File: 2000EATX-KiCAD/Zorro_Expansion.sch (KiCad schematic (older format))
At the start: 119 parts, among them CN601 Amiga-2000-Zorro-Slot, CN602 Amiga-2000-Zorro-Slot, CN603 Amiga-2000-Zorro-Slot, CN604 Amiga-2000-Zorro-Slot, CN605 Amiga-2000-Zorro-Slot, U606 74LS32

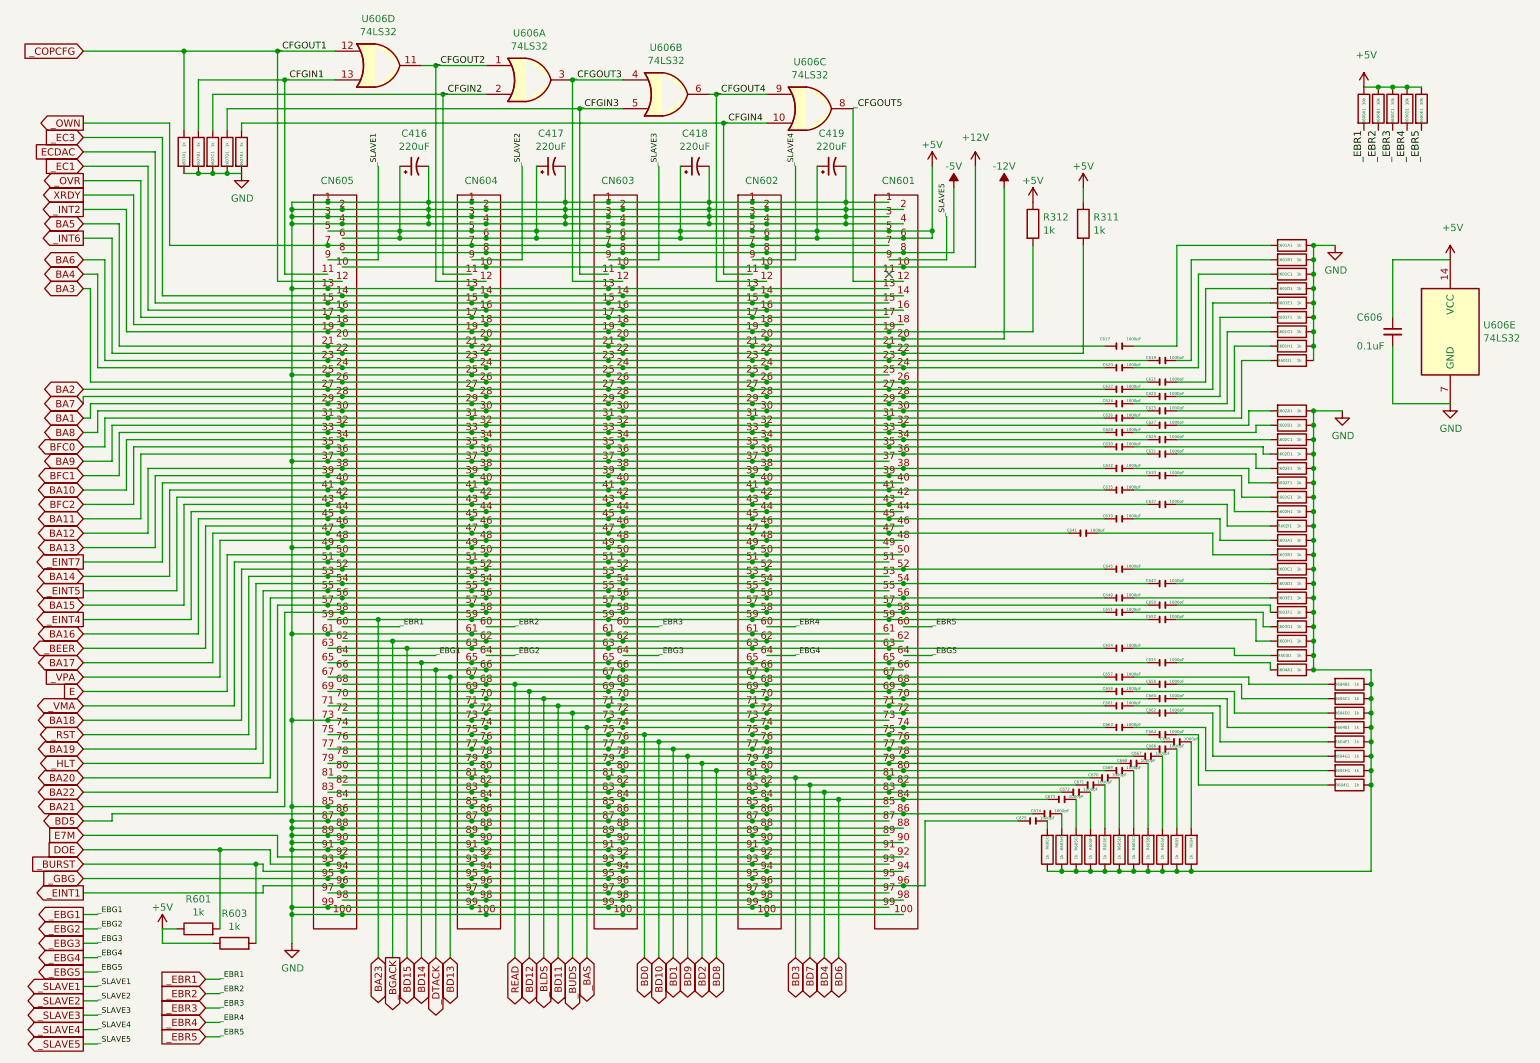
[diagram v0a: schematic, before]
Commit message: Add files via upload
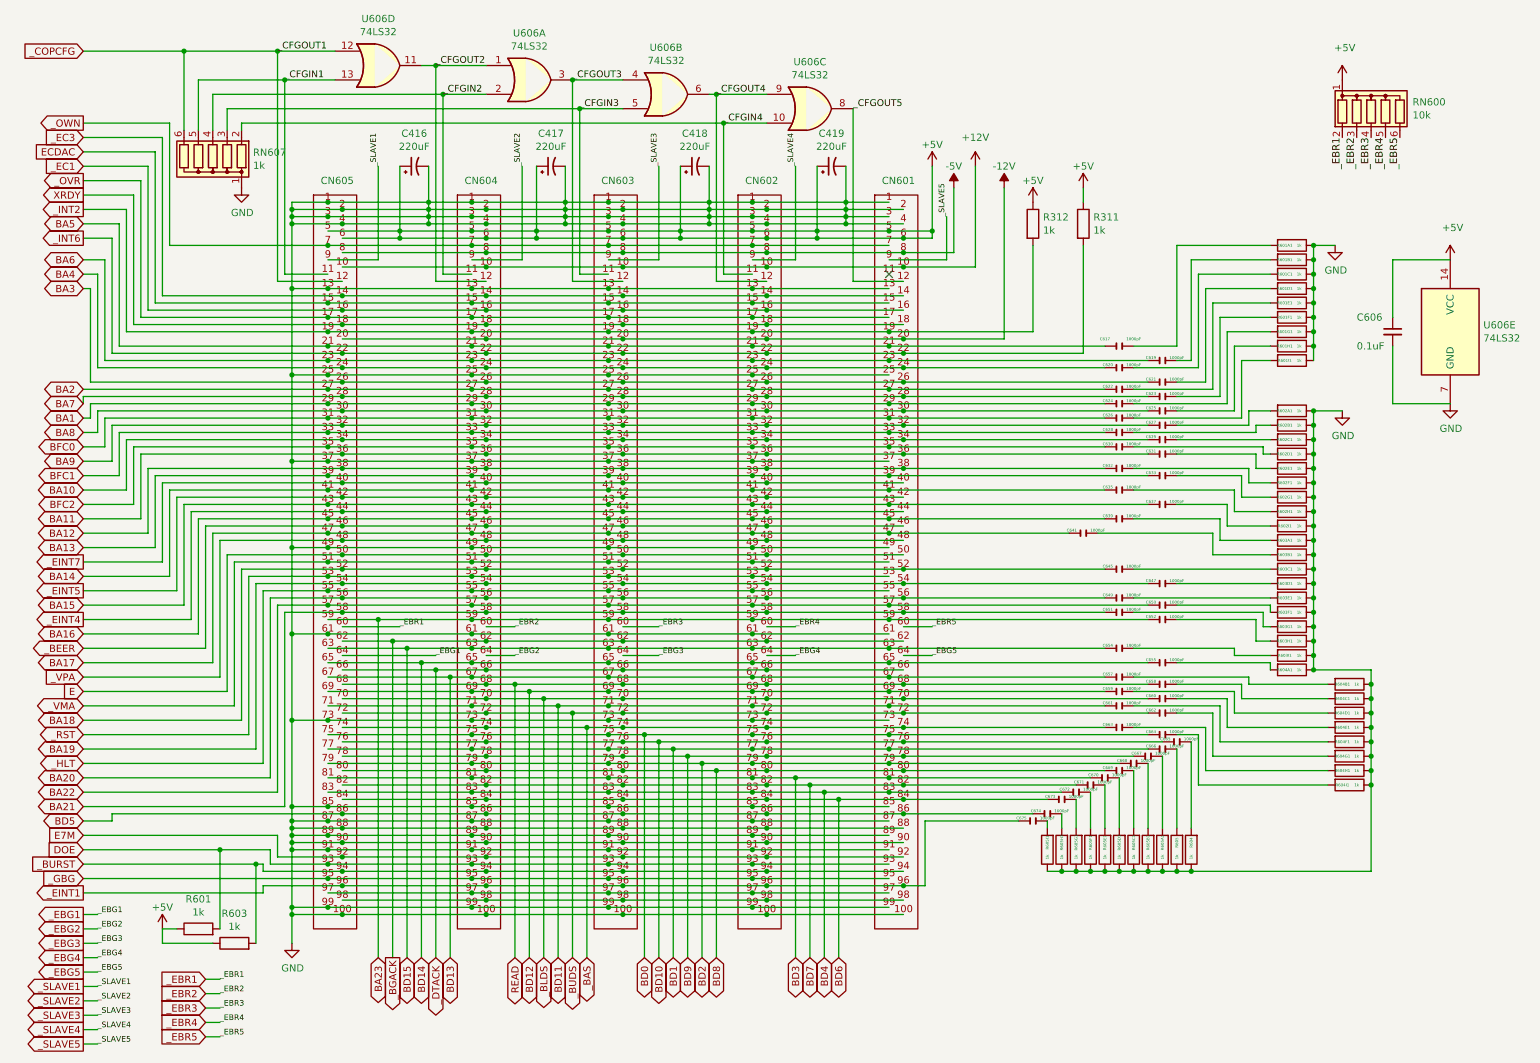
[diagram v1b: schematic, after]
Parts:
- removed R600A1, R600B1, R600C1, R600D1, R600E1: 10k, Resistor_SMD:R_1206_3216Metric, symbol Device:R
- removed R607A1, R607B1, R607C1, R607D1, R607E1: 1k, Resistor_SMD:R_1206_3216Metric, symbol Device:R
- added RN600: 10k, Resistor_THT:R_Array_SIP6, symbol Device:R_Network05
- added RN607: 1k, Resistor_THT:R_Array_SIP6, symbol Device:R_Network05
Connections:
- net +5V: now also RN600.1 (common)
- net GND: now also RN607.1 (common)
- net _CFGIN1: now also RN607.5 (R4)
- net _CFGIN2: now also RN607.4 (R3)
- net _CFGIN3: now also RN607.3 (R2)
- net _CFGIN4: now also RN607.2 (R1)
- net _COPCFG: now also RN607.6 (R5)
- net _EBR1: now also RN600.2 (R1)
- net _EBR2: now also RN600.3 (R2)
- net _EBR3: now also RN600.4 (R3)
- net _EBR4: now also RN600.5 (R4)
- net _EBR5: now also RN600.6 (R5)
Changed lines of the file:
@@
 EELAYER 30 0
 EELAYER END
-$Descr A4 11693 8268
+$Descr B 17000 11000
 encoding utf-8
 Sheet 2 13
@@
 Text GLabel 1050 750  0    50   Input ~ 0
 _COPCFG
-$Comp
-L power:GND #PWR0151
-U 1 1 60529FF3
-P 2150 1600
-F 0 "#PWR0151" H 2150 1350 50  0001 C CNN
-F 1 "GND" H 2155 1427 50  0000 C CNN
-F 2 "" H 2150 1600 50  0001 C CNN
-F 3 "" H 2150 1600 50  0001 C CNN
-	1    2150 1600
-	1    0    0    -1
-$EndComp
 Wire Wire Line
 	1750 1300 1750 750
@@
 	2250 6400 1050 6400
 $Comp
-L power:+5V #PWR0162
-U 1 1 73C05A53
-P 9950 1000
-F 0 "#PWR0162" H 9950 850 50  0001 C CNN
-F 1 "+5V" H 9967 1223 50  0000 C CNN
-F 2 "" H 9950 1000 50  0001 C CNN
-F 3 "" H 9950 1000 50  0001 C CNN
-	1    9950 1000
-	1    0    0    -1
-$EndComp
-Text Label 9950 1300 3    51   ~ 0
-_EBR1
-Text Label 10050 1300 3    51   ~ 0
-_EBR2
-Text Label 10150 1300 3    51   ~ 0
-_EBR3
-Text Label 10250 1300 3    51   ~ 0
-_EBR4
-Text Label 10350 1300 3    51   ~ 0
-_EBR5
-$Comp
 L 74xx:74LS32 U606
 U 5 1 73D576B9
@@
 $EndComp
 $Comp
-L Device:R R604G1
-U 1 1 7568AC17
-P 9850 5650
-F 0 "R604G1" V 9850 5600 20  0000 C CNN
-F 1 "1k" V 9850 5700 20  0000 C CNN
-F 2 "Resistor_SMD:R_1206_3216Metric" V 9780 5650 50  0001 C CNN
-F 3 "~" H 9850 5650 50  0001 C CNN
-	1    9850 5650
-	0    1    1    0
-$EndComp
-$Comp
 L Device:R R604H1
 U 1 1 7568B190
@@
 Wire Wire Line
 	10000 5550 10000 5450
-Connection ~ 10000 5650
-Wire Wire Line
-	10000 5650 10000 5550
 Connection ~ 10000 5750
-Wire Wire Line
-	10000 5750 10000 5650
 Connection ~ 9600 5050
 $Comp
@@
 	8750 6450 10000 6450
 Connection ~ 10000 5850
-$Comp
-L Device:R R600A1
-U 1 1 77C6BDFF
-P 9950 1150
-F 0 "R600A1" V 9950 1100 20  0000 C CNN
-F 1 "10k" V 9950 1200 20  0000 C CNN
-F 2 "Resistor_SMD:R_1206_3216Metric" V 9880 1150 50  0001 C CNN
-F 3 "~" H 9950 1150 50  0001 C CNN
-	1    9950 1150
-	1    0    0    -1
-$EndComp
-$Comp
-L Device:R R600B1
-U 1 1 77C6D385
-P 10050 1150
-F 0 "R600B1" V 10050 1100 20  0000 C CNN
-F 1 "10k" V 10050 1200 20  0000 C CNN
-F 2 "Resistor_SMD:R_1206_3216Metric" V 9980 1150 50  0001 C CNN
-F 3 "~" H 10050 1150 50  0001 C CNN
-	1    10050 1150
-	1    0    0    -1
-$EndComp
-$Comp
-L Device:R R600C1
-U 1 1 77C6D685
-P 10150 1150
-F 0 "R600C1" V 10150 1100 20  0000 C CNN
-F 1 "10k" V 10150 1200 20  0000 C CNN
-F 2 "Resistor_SMD:R_1206_3216Metric" V 10080 1150 50  0001 C CNN
-F 3 "~" H 10150 1150 50  0001 C CNN
-	1    10150 1150
-	1    0    0    -1
-$EndComp
-$Comp
-L Device:R R600D1
-U 1 1 77C6D806
-P 10250 1150
-F 0 "R600D1" V 10250 1100 20  0000 C CNN
-F 1 "10k" V 10250 1200 20  0000 C CNN
-F 2 "Resistor_SMD:R_1206_3216Metric" V 10180 1150 50  0001 C CNN
-F 3 "~" H 10250 1150 50  0001 C CNN
-	1    10250 1150
-	1    0    0    -1
-$EndComp
-$Comp
-L Device:R R600E1
-U 1 1 77C6D9DF
-P 10350 1150
-F 0 "R600E1" V 10350 1100 20  0000 C CNN
-F 1 "10k" V 10350 1200 20  0000 C CNN
-F 2 "Resistor_SMD:R_1206_3216Metric" V 10280 1150 50  0001 C CNN
-F 3 "~" H 10350 1150 50  0001 C CNN
-	1    10350 1150
-	1    0    0    -1
-$EndComp
-Wire Wire Line
-	9950 1000 10050 1000
-Connection ~ 10050 1000
-Wire Wire Line
-	10050 1000 10150 1000
-Connection ~ 10150 1000
-Wire Wire Line
-	10150 1000 10250 1000
-Connection ~ 10250 1000
-Wire Wire Line
-	10250 1000 10350 1000
-$Comp
-L Device:R R607A1
-U 1 1 77DA0D4E
-P 1750 1450
-F 0 "R607A1" V 1750 1400 20  0000 C CNN
-F 1 "1k" V 1750 1500 20  0000 C CNN
-F 2 "Resistor_SMD:R_1206_3216Metric" V 1680 1450 50  0001 C CNN
-F 3 "~" H 1750 1450 50  0001 C CNN
-	1    1750 1450
-	1    0    0    -1
-$EndComp
-$Comp
-L Device:R R607B1
-U 1 1 77DACF10
-P 1850 1450
-F 0 "R607B1" V 1850 1400 20  0000 C CNN
-F 1 "1k" V 1850 1500 20  0000 C CNN
-F 2 "Resistor_SMD:R_1206_3216Metric" V 1780 1450 50  0001 C CNN
-F 3 "~" H 1850 1450 50  0001 C CNN
-	1    1850 1450
-	1    0    0    -1
-$EndComp
-$Comp
-L Device:R R607C1
-U 1 1 77DAD45F
-P 1950 1450
-F 0 "R607C1" V 1950 1400 20  0000 C CNN
-F 1 "1k" V 1950 1500 20  0000 C CNN
-F 2 "Resistor_SMD:R_1206_3216Metric" V 1880 1450 50  0001 C CNN
-F 3 "~" H 1950 1450 50  0001 C CNN
-	1    1950 1450
-	1    0    0    -1
-$EndComp
-$Comp
-L Device:R R607D1
-U 1 1 77DAD92E
-P 2050 1450
-F 0 "R607D1" V 2050 1400 20  0000 C CNN
-F 1 "1k" V 2050 1500 20  0000 C CNN
-F 2 "Resistor_SMD:R_1206_3216Metric" V 1980 1450 50  0001 C CNN
-F 3 "~" H 2050 1450 50  0001 C CNN
-	1    2050 1450
-	1    0    0    -1
-$EndComp
-$Comp
-L Device:R R607E1
-U 1 1 77DADE67
-P 2150 1450
-F 0 "R607E1" V 2150 1400 20  0000 C CNN
-F 1 "1k" V 2150 1500 20  0000 C CNN
-F 2 "Resistor_SMD:R_1206_3216Metric" V 2080 1450 50  0001 C CNN
-F 3 "~" H 2150 1450 50  0001 C CNN
-	1    2150 1450
-	1    0    0    -1
-$EndComp
-Wire Wire Line
-	1750 1600 1850 1600
-Connection ~ 1850 1600
-Wire Wire Line
-	1850 1600 1950 1600
-Connection ~ 1950 1600
-Wire Wire Line
-	1950 1600 2050 1600
-Connection ~ 2050 1600
-Wire Wire Line
-	2050 1600 2150 1600
 Wire Wire Line
 	8350 5200 9050 5200
@@
 Wire Wire Line
 	8550 6150 8550 5650
+$Comp
+L Device:R_Network05 RN600
+U 1 1 607C60FC
+P 10000 1150
+F 0 "RN600" H 10288 1196 50  0000 L CNN
+F 1 "10k" H 10288 1105 50  0000 L CNN
+F 2 "Resistor_THT:R_Array_SIP6" V 10375 1150 50  0001 C CNN
+F 3 "http://www.vishay.com/docs/31509/csc.pdf" H 10000 1150 50  0001 C CNN
+	1    10000 1150
+	1    0    0    -1
+$EndComp
+Text Label 10200 1350 3    51   ~ 0
+_EBR5
+Text Label 10100 1350 3    51   ~ 0
+_EBR4
+Text Label 10000 1350 3    51   ~ 0
+_EBR3
+Text Label 9900 1350 3    51   ~ 0
+_EBR2
+Text Label 9800 1350 3    51   ~ 0
+_EBR1
+$Comp
+L power:+5V #PWR0162
+U 1 1 73C05A53
+P 9800 950
+F 0 "#PWR0162" H 9800 800 50  0001 C CNN
+F 1 "+5V" H 9817 1173 50  0000 C CNN
+F 2 "" H 9800 950 50  0001 C CNN
+F 3 "" H 9800 950 50  0001 C CNN
+	1    9800 950
+	1    0    0    -1
+$EndComp
+$Comp
+L Device:R R604G1
+U 1 1 7568AC17
+P 9850 5650
+F 0 "R604G1" V 9850 5600 20  0000 C CNN
+F 1 "1k" V 9850 5700 20  0000 C CNN
+F 2 "Resistor_SMD:R_1206_3216Metric" V 9780 5650 50  0001 C CNN
+F 3 "~" H 9850 5650 50  0001 C CNN
+	1    9850 5650
+	0    1    1    0
+$EndComp
+Wire Wire Line
+	10000 5550 10000 5650
+Connection ~ 10000 5650
+Wire Wire Line
+	10000 5650 10000 5750
+$Comp
+L Device:R_Network05 RN607
+U 1 1 6106B5AE
+P 1950 1500
+F 0 "RN607" H 1670 1454 50  0000 R CNN
+F 1 "1k" H 1670 1545 50  0000 R CNN
+F 2 "Resistor_THT:R_Array_SIP6" V 2325 1500 50  0001 C CNN
+F 3 "http://www.vishay.com/docs/31509/csc.pdf" H 1950 1500 50  0001 C CNN
+	1    1950 1500
+	-1   0    0    1
+$EndComp
+$Comp
+L power:GND #PWR?
+U 1 1 612D942C
+P 2150 1700
+F 0 "#PWR?" H 2150 1450 50  0001 C CNN
+F 1 "GND" H 2155 1527 50  0000 C CNN
+F 2 "" H 2150 1700 50  0001 C CNN
+F 3 "" H 2150 1700 50  0001 C CNN
+	1    2150 1700
+	1    0    0    -1
+$EndComp
 $EndSCHEMATC
